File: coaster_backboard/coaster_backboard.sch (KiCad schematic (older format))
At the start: 83 parts, among them J1 USB, P1 TC2030, U1 STM32F072C8Tx, U2 IS31FL3733-QF

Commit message: routing 80%
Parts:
- added C11, C12, C13, C14, C15, C16, C17, C18, C19, C20: 100n, otter:C_0402, symbol Device:C_Small
- added J2, J3, J4, J5: MP, Connector_Pin:Pin_D1.0mm_L10.0mm_LooseFit, symbol Connector:Conn_01x01_Female
- added J6, J7: Solderpad, Connector_Pin:Pin_D0.7mm_L6.5mm_W1.8mm_FlatFork, symbol Connector:Conn_01x01_Female
- added J8: USB, otter:918-418K2022Y40004, symbol Connector:USB_C_Receptacle
- added JP1: DFU, otter:R_0805, symbol Device:Jumper
- added R10, R11, R14, R15, R5, R6, R7, R8, R9: 5k1, otter:R_0402, symbol Device:R_Small
- added TH1: NTC, otter:R_0603, symbol Device:Thermistor_NTC
- added U?: MCP1700-3302E_SOT23, Package_TO_SOT_SMD:SOT-23, symbol Regulator_Linear:MCP1700-3302E_SOT23
- gave numbers to parts that had none: 39
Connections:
- net +3V3: now also C12.1, C14.1, C15.1, C16.1, C17.1, C18.1, JP1.2, R10.2, R6.1, R7.2, R8.2, U?.2 (VO)
- net D+: now also U1.33 (PA12), J8.A6 (D+), J8.B6 (D+)
- net D-: now also U1.32 (PA11), J8.A7 (D-), J8.B7 (D-)
- net GND: now also C11.2, C12.2, C13.2, C14.2, C15.2, C16.2, C17.2, C18.2, C19.2, C20.2, J7.1 (Pin_1), J8.A1 (GND), J8.A12 (GND), J8.B1 (GND), J8.B12 (GND), J8.S1 (SHIELD), R11.2, R14.1, R15.2, R5.1, R9.2, TH1.2, U?.1 (GND)
- net INT: now also U1.26 (PB13)
- net SCL: now also U1.42 (PB6), R6.2
- net SDA: now also U1.43 (PB7), R7.1
- net SDB: now also U1.27 (PB14)
- net SWCLK: now also U1.37 (PA14)
- net SWDIO: now also U1.34 (PA13)
- net VBUS: now also C11.1, J8.A4 (VBUS), J8.A9 (VBUS), J8.B4 (VBUS), J8.B9 (VBUS), U?.3 (VI)
- net NTC1: now reaches U1.10 (PA0)
- net NTC1: now also C19.1, J6.1 (Pin_1), R8.1, R9.1
- net NTC0: now reaches U1.11 (PA1)
- net NTC0: now also C20.1, R10.1, R11.1, TH1.1
- net at U1.44 (BOOT0): now also JP1.1, R5.2
- net at U1.7 (NRST): now also C13.1
- new net: J8.A5 (CC1), R14.2
- new net: J8.B5 (CC2), R15.1
- no-connect marks 1 -> 19
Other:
- moved on the sheet: C1, C10, C2, C3, C4, C5, C6, C7, C8, C9, D1, D10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

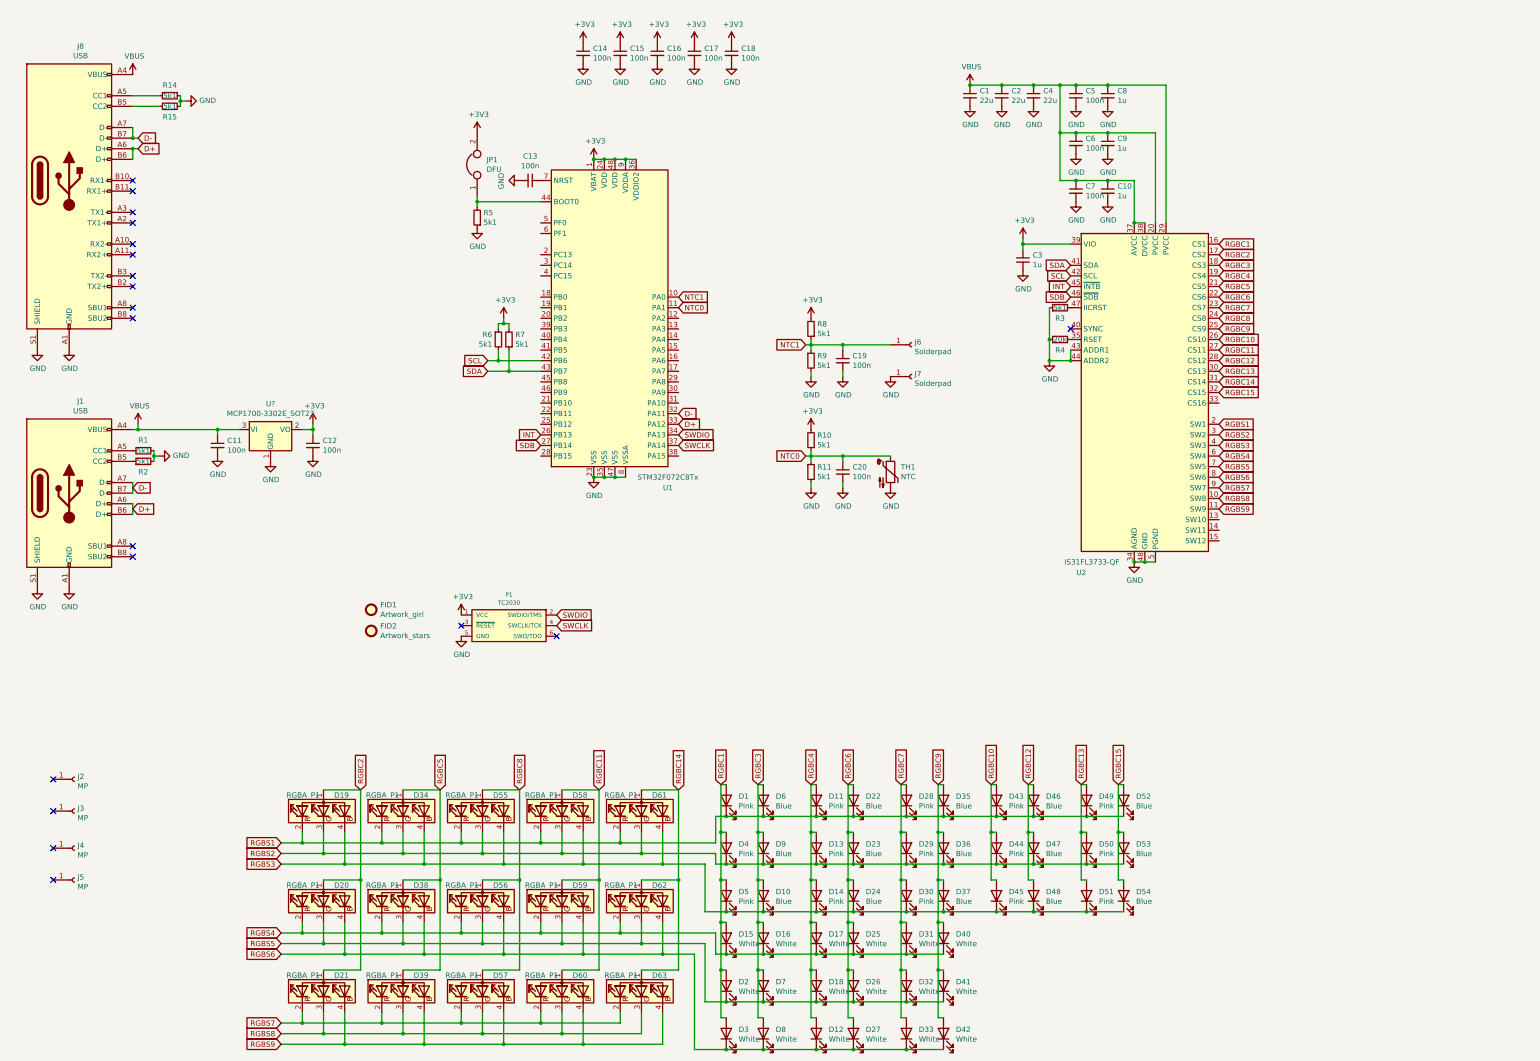
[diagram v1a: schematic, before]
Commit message: updated hw
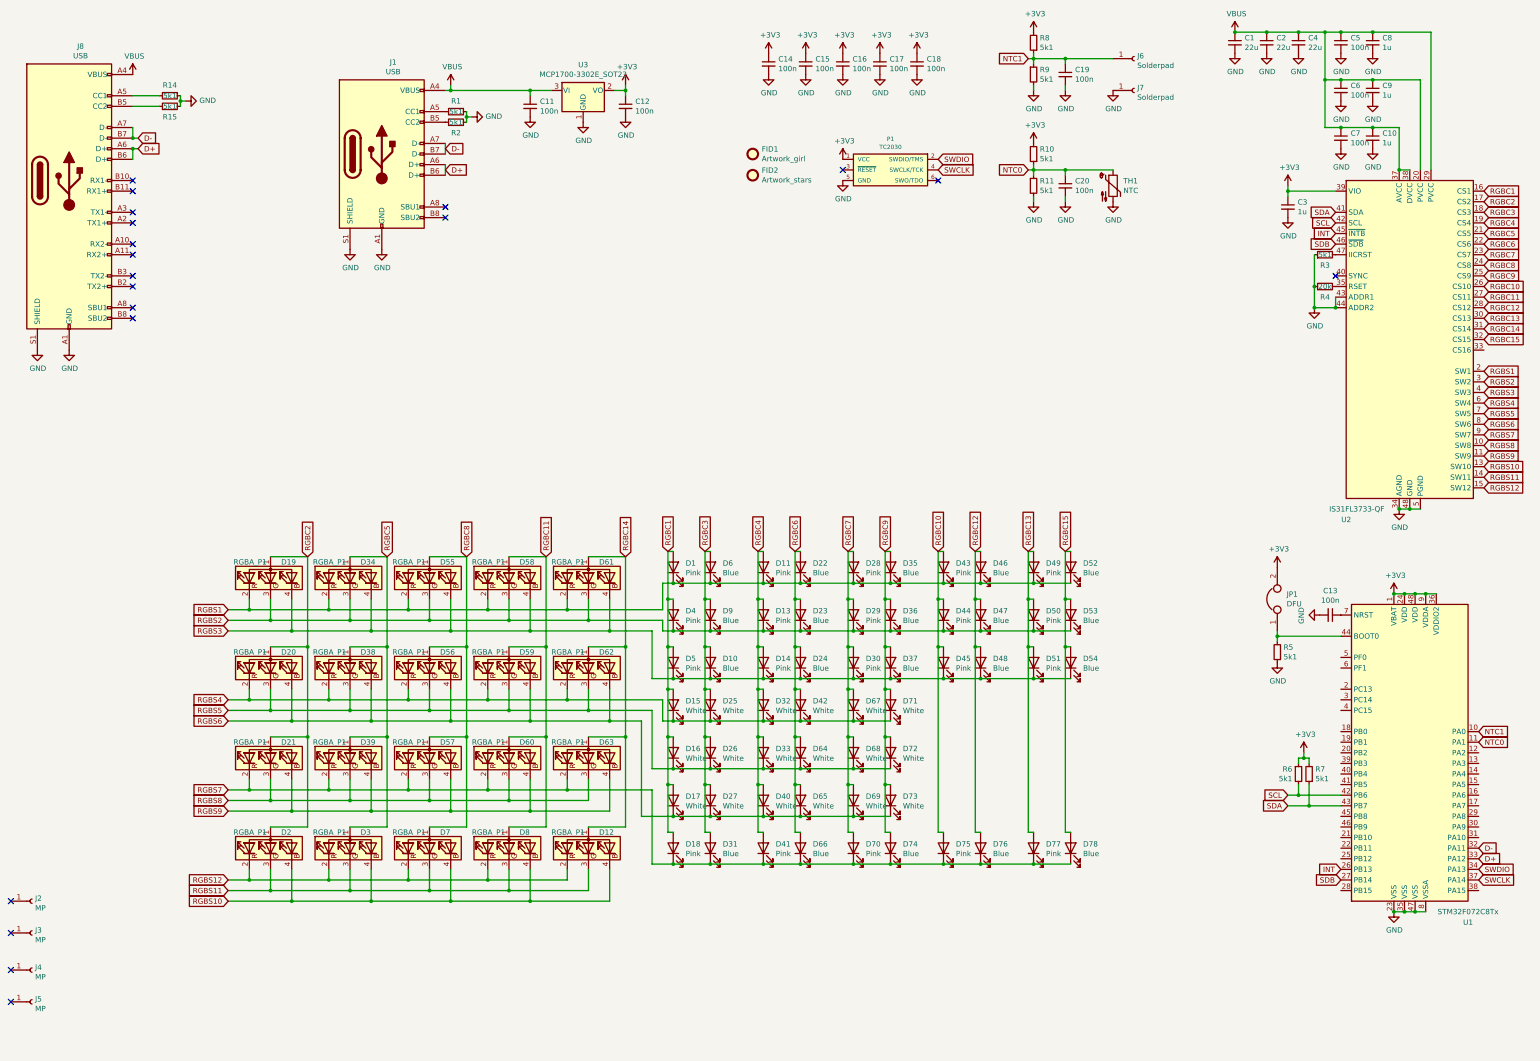
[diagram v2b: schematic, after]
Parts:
- removed D12, D2, D3, D7, D8: White, LED_SMD:LED_0603_1608Metric, symbol Device:LED
- added D12, D2, D3, D7, D8: RGBA_P1, otter:FC-B1010RGBT-HG, symbol otter:RGBA_P1
- added D64, D65, D67, D68, D69, D71, D72, D73: White, LED_SMD:LED_0603_1608Metric, symbol Device:LED
- added D66, D74, D76, D78: Blue, LED_SMD:LED_0603_1608Metric, symbol Device:LED
- added D70, D75, D77: Pink, LED_SMD:LED_0603_1608Metric, symbol Device:LED
- D18, D41: value White -> Pink
- D31: value White -> Blue
- J1: footprint otter:USB-C 16Pin -> otter:USB-C 16Pin InBoard
- gave numbers to parts that had none: 1
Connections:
- net RGBC1: now also D16.2 (A), D17.2 (A), D18.2 (A)
- net RGBC10: now also D75.2 (A)
- net RGBC11: now also D8.1 (A)
- net RGBC12: now also D76.2 (A)
- net RGBC13: now also D77.2 (A)
- net RGBC14: now also D12.1 (A)
- net RGBC15: now also D78.2 (A)
- net RGBC2: now also D2.1 (A)
- net RGBC3: now also D25.2 (A), D26.2 (A), D27.2 (A), D31.2 (A); no longer D16.2 (A)
- net RGBC4: now also D32.2 (A), D33.2 (A), D40.2 (A), D41.2 (A); no longer D17.2 (A), D18.2 (A)
- net RGBC5: now also D3.1 (A)
- net RGBC6: now also D42.2 (A), D64.2 (A), D65.2 (A), D66.2 (A); no longer D25.2 (A), D26.2 (A), D27.2 (A)
- net RGBC7: now also D67.2 (A), D68.2 (A), D69.2 (A), D70.2 (A); no longer D31.2 (A), D32.2 (A), D33.2 (A)
- net RGBC8: now also D7.1 (A)
- net RGBC9: now also D71.2 (A), D72.2 (A), D73.2 (A), D74.2 (A); no longer D40.2 (A), D41.2 (A), D42.2 (A)
- net RGBS4: now also D32.1 (K), D42.1 (K), D67.1 (K), D71.1 (K); no longer D16.1 (K), D17.1 (K), D31.1 (K), D40.1 (K)
- net RGBS5: now also D16.1 (K), D33.1 (K), D64.1 (K), D68.1 (K), D72.1 (K); no longer D18.1 (K), D32.1 (K), D41.1 (K)
- net RGBS6: now also D17.1 (K), D40.1 (K), D65.1 (K), D69.1 (K), D73.1 (K); no longer D33.1 (K), D42.1 (K)
- net RGBS7: now also D18.1 (K), D31.1 (K), D41.1 (K), D66.1 (K), D70.1 (K), D74.1 (K), D75.1 (K), D76.1 (K), D77.1 (K), D78.1 (K)
- net RGBS10: now reaches U2.13 (SW10)
- net RGBS10: now also D12.4 (BK), D2.4 (BK), D3.4 (BK), D7.4 (BK), D8.4 (BK)
- net RGBS11: now reaches U2.14 (SW11)
- net RGBS11: now also D12.3 (GK), D2.3 (GK), D3.3 (GK), D7.3 (GK), D8.3 (GK)
- net RGBS12: now reaches U2.15 (SW12)
- net RGBS12: now also D12.2 (RK), D2.2 (RK), D3.2 (RK), D7.2 (RK), D8.2 (RK)
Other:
- moved on the sheet: C1, C10, C11, C12, C13, C14, C15, C16, C17, C18, C19, C2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
